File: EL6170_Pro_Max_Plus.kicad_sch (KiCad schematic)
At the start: 117 parts, among them CN1 PJ-327A0-SMT, J1 USB_C_Receptacle, J2 microSD, Q1 MMBT3904, Q2 MMBT3904, Q3 2N7002, Q4 AO3401A, Q5 AO3401A, SW1 SW_Push, U1 ESP32-S3, U10 ME6211C33M5, U11 TP5400_C2891434, U2 TPS61040DBV, U3 ESP-PSRAM64H, U4 W25Q128JVS, U5 ME6217C33M5, U6 CH340K, U7 RFANT5220110A0T, U8 CH334R, U9 PCM5102A, X1 40MHz, X2 12MHz

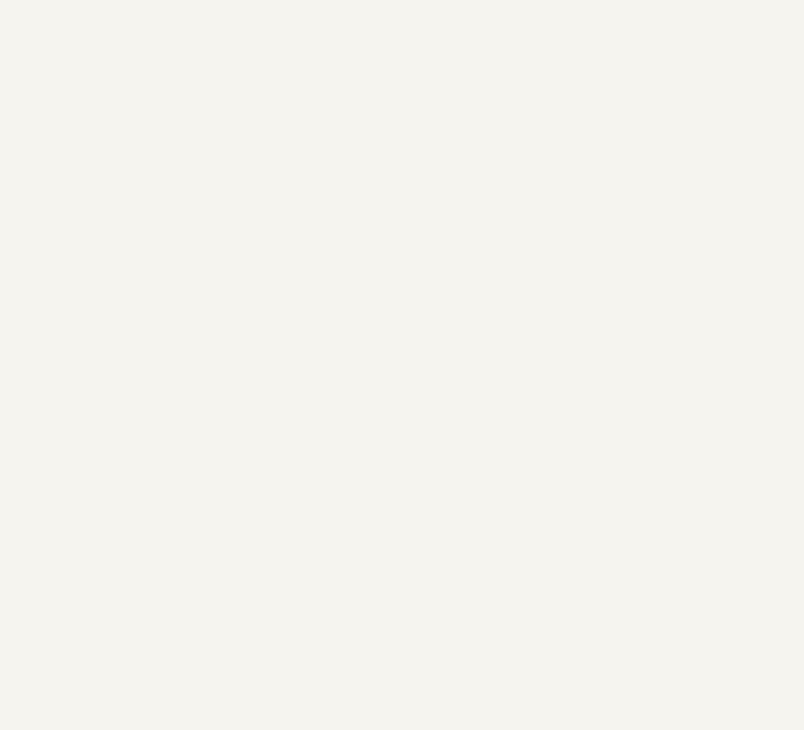
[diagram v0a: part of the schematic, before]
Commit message: sync
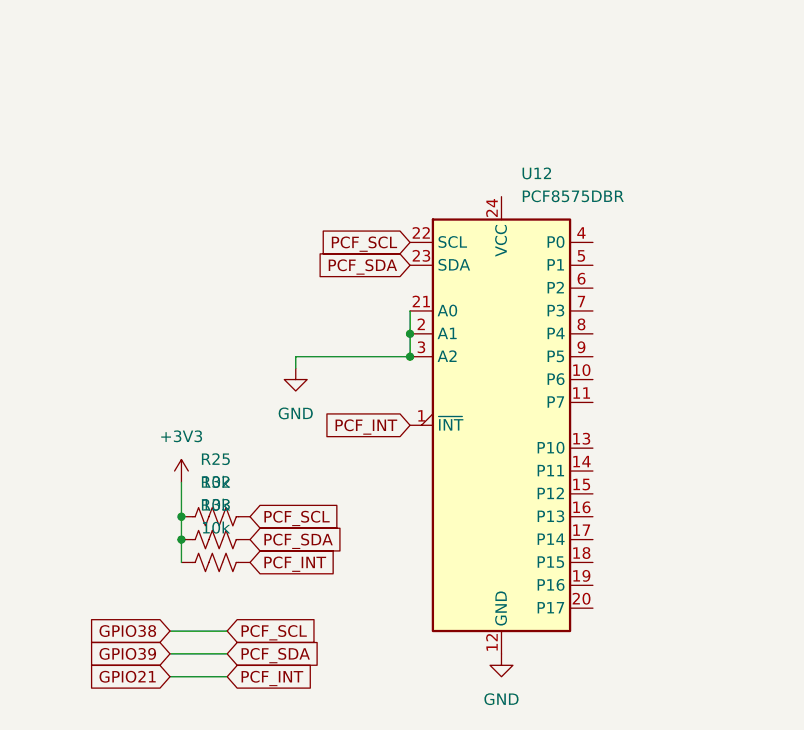
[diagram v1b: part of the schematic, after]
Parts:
- added R25, R32, R33: 10k, SparkFun-Resistor:R_0402_1005Metric, symbol SparkFun-Resistor:10k_0402
- added U12: PCF8575DBR, Package_SO:SSOP-24_5.3x8.2mm_P0.65mm, symbol Interface_Expansion:PCF8575DBR
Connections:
- net +3V3: now also R25.1, R32.1, R33.1
- net GND: now also U12.12 (GND), U12.2 (A1), U12.21 (A0), U12.3 (A2)
- net GPIO21: now also R33.2, U12.1 (~{INT})
- net GPIO38: now also R25.2, U12.22 (SCL)
- net GPIO39: now also R32.2, U12.23 (SDA)
